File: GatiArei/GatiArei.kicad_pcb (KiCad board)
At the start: 2 copper layers, 40 parts, among them J1 LCD_PORT, J2 RFID_PORT, P1 USB_C_Plug_USB2.0, Q1 S8050, Q2 S8050, SW1 SW1, SW2 SW1, U1 MCP1700-3302E_SOT23, U2 CP2102N-A01-GQFN24, U3 ESP32-WROOM-32

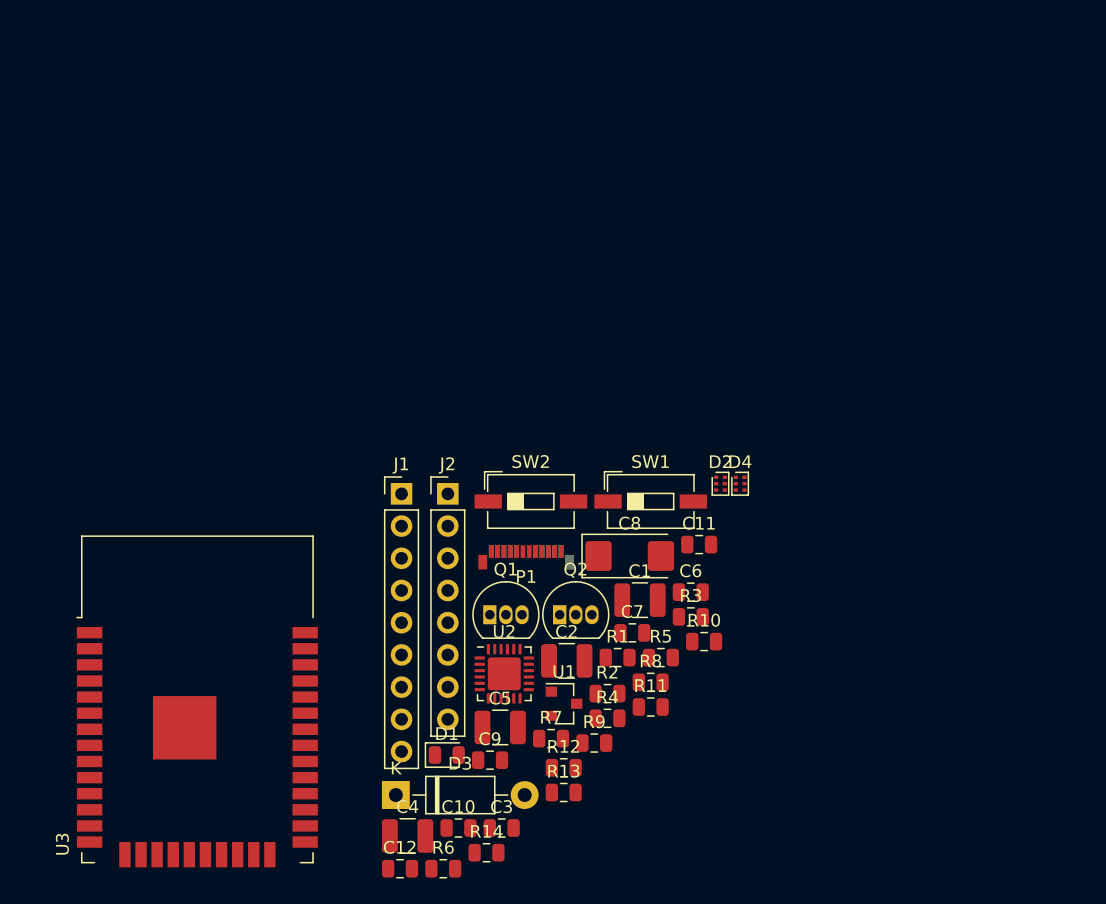
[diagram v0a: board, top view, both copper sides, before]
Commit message: Adding PCB design
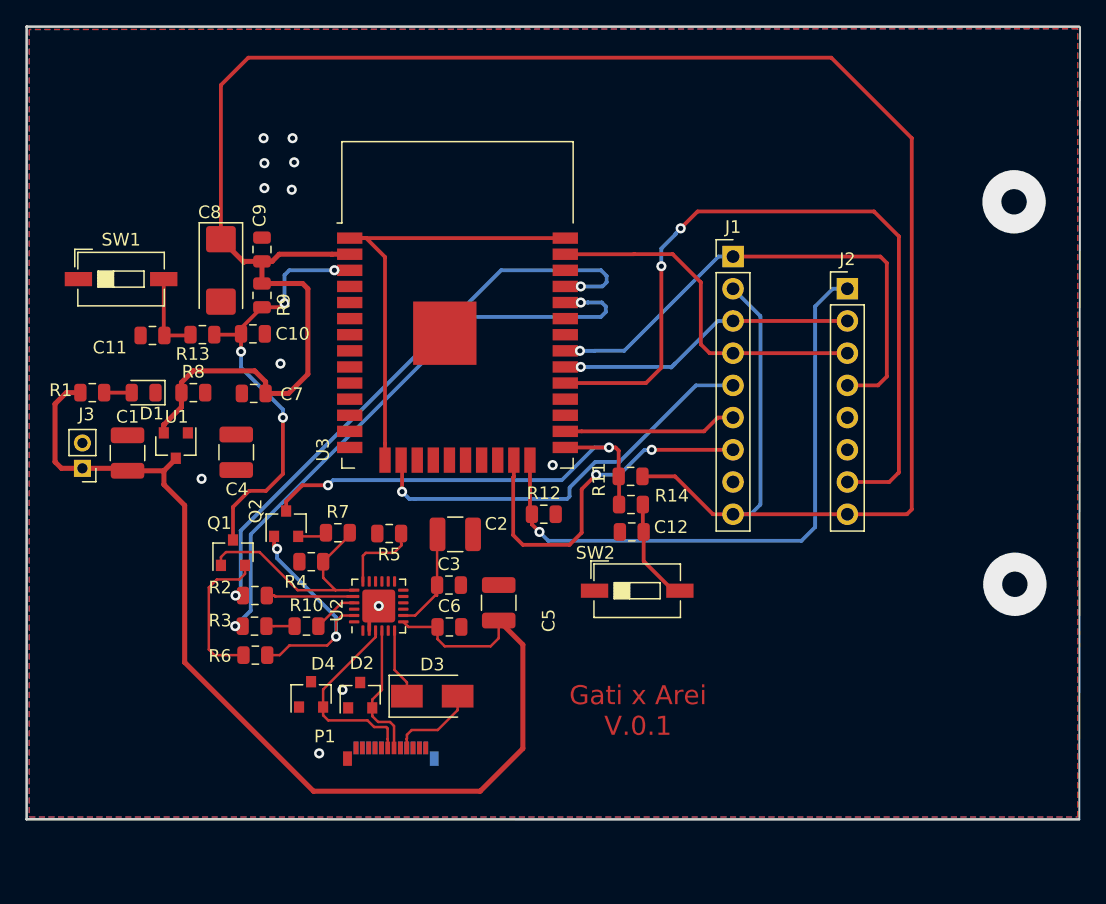
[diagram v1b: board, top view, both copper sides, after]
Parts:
- added J3: Bat_Con, Connector_PinHeader_2.00mm:PinHeader_1x02_P2.00mm_Vertical, F.Cu at (21.4, 120.3)
- D2, D4: value PESD5V0L4UF -> ESD5V; footprint Package_TO_SOT_SMD:SOT-886 -> Package_TO_SOT_SMD:SOT-23
- D3: footprint Diode_THT:D_DO-41_SOD81_P10.16mm_Horizontal -> Diode_SMD:D_SMA
- P1: value USB_C_Plug_USB2.0 -> USB_C
- Q1, Q2: footprint Package_TO_SOT_THT:TO-92_Inline -> Package_TO_SOT_SMD:SOT-23
- U1: value MCP1700-3302E_SOT23 -> MCP1700
- U2: value CP2102N-A01-GQFN24 -> CP2102N
- moved R1 46.4 mm to (22.2, 114.4)
- moved C11 46.2 mm to (26.9, 109.9), turned to 180 degrees
- moved R13 46.0 mm to (30.9, 109.8), turned to 180 degrees
- moved SW1 45.3 mm to (24.4, 105.4)
- moved C9 44.1 mm to (35.6, 103.1), turned to 90 degrees
- moved R9 44.0 mm to (35.6, 106.7), turned to 270 degrees
- moved R8 42.7 mm to (30.1, 114.4)
- moved C10 42.2 mm to (34.8, 109.7)
- moved C1 42.0 mm to (25.0, 119.1), turned to 90 degrees
- moved C8 39.3 mm to (32.3, 104.7), turned to 270 degrees
- moved D4 37.7 mm to (39.4, 138.2), turned to 90 degrees
- moved U3 37.3 mm to (51.0, 110.4)
- moved D1 37.3 mm to (26.2, 114.4), turned to 180 degrees
- moved U1 36.8 mm to (28.8, 118.5), turned to 270 degrees
- moved J2 35.4 mm to (81.7, 106.2)
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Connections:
- C10 pad 1: Net-(C10-Pad1) -> EN
- R11 pad 2: Net-(R11-Pad2) -> IO0
- R9 pad 2: Net-(C10-Pad1) -> EN
- U3 pad 25: Net-(R11-Pad2) -> IO0
- U3 pad 3: Net-(C10-Pad1) -> EN
- U3 pad 34: Net-(U3-Pad34) -> RXD0
- U3 pad 35: Net-(U3-Pad35) -> TXD0
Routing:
- net VDD_ESP: track 0.00 -> 182.7 mm
- net VDD_REGIN: track 0.00 -> 100.4 mm
- net RFID_RST: track 0.00 -> 61.3 mm, vias 0 -> 2
- net RFID_SS: track 0.00 -> 49.0 mm, vias 0 -> 1
- net RXD0: track 0.00 -> 47.6 mm, vias 0 -> 2
- net TXD0: track 0.00 -> 47.3 mm, vias 0 -> 2
- net SPI_MISO: track 0.00 -> 41.0 mm, vias 0 -> 1
- net IO0: track 0.00 -> 36.6 mm, vias 0 -> 2
- net Net-(U3-Pad1): track 0.00 -> 36.4 mm
- net EN: track 0.00 -> 34.9 mm, vias 0 -> 4
- net LCD_DC: track 0.00 -> 33.0 mm, vias 0 -> 1
- net LCD_SS: track 0.00 -> 28.7 mm, vias 0 -> 2
- net SPI_MOSI: track 0.00 -> 28.3 mm
- net SPI_SCK: track 0.00 -> 24.2 mm, vias 0 -> 1
- net DTR: track 0.00 -> 18.8 mm, vias 0 -> 2
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- added copper zone on B.Cu, net GND
- added copper zone on F.Cu, net GND
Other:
- board outline added: 83.1 x 62.5 mm
- board text added: "Gati x Arei V.0.1"
